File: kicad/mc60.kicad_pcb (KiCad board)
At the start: 2 copper layers, 60 x 70 mm, 108 parts, among them CN1 Conn_GPS, CN2 Conn_GNSS, CN3 SD_CARD, CN4 SIM_Card, CN5 Audio-Jack-4, CN6 5V_IN, J1 B_LS_N, J2 B_VRTC, J3 B_SPKP, J4 B_SPKN, J5 B_ADC, Q1 DTC114E, Q2 DTC114E, Q3 DTC114E, Q4 DTC143ZUA, U1 MC60_0, U2 TXB0108PWR, U3 MIC29302, U4 LP5907-3V3, U5 LP5907-2V8

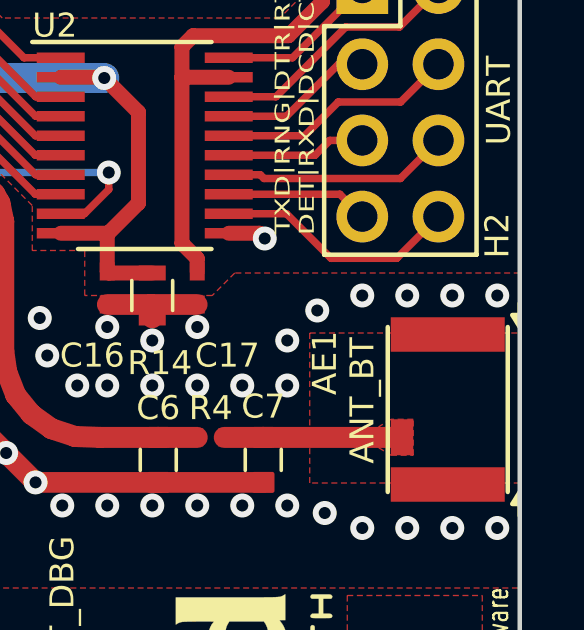
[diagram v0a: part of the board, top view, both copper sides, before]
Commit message: layout wip
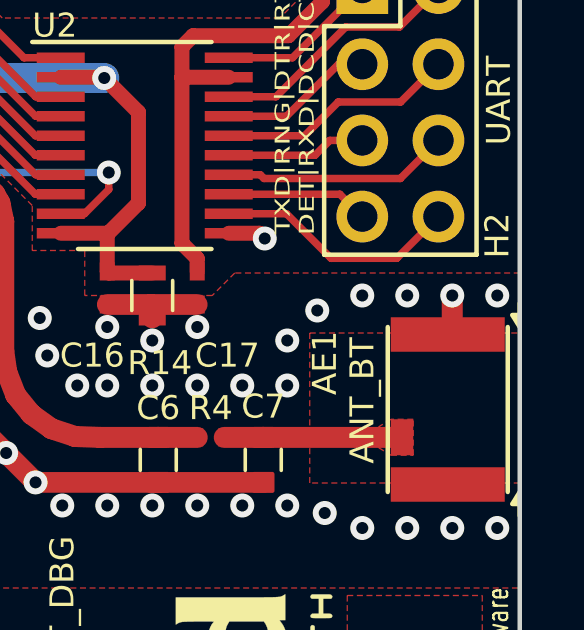
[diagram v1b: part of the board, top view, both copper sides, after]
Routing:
- net GND: track 272.8 -> 274.1 mm
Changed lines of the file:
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@@
-(kicad_pcb (version 20171130) (host pcbnew 5.0.0-rc2-dev-unknown-5d71153~64~ubuntu17.10.1)
+(kicad_pcb (version 20171130) (host pcbnew 5.0.0-rc2-dev-unknown-c8a7840~64~ubuntu16.04.1)
   (general
     (thickness 1.6)
     (drawings 25)
-    (tracks 1046)
+    (tracks 1048)
     (zones 0)
     (modules 108)
@@
     (0 F.Cu signal)
     (31 B.Cu signal)
-    (32 B.Adhes user hide)
-    (33 F.Adhes user hide)
+    (32 B.Adhes user)
+    (33 F.Adhes user)
     (34 B.Paste user hide)
     (35 F.Paste user hide)
     (36 B.SilkS user)
     (37 F.SilkS user)
-    (38 B.Mask user hide)
+    (38 B.Mask user)
     (39 F.Mask user)
     (40 Dwgs.User user)
@@
       (effects (font (size 0.8 0.8) (thickness 0.12)) (justify mirror))
     )
-    (fp_text value B_LS_N (at 0 -3.5 -90) (layer B.SilkS)
+    (fp_text value B_LS_N (at 0 -3.5 90) (layer B.SilkS)
       (effects (font (size 0.8 0.8) (thickness 0.12)) (justify mirror))
     )
@@
   (via (at 92.25 112.25) (size 0.7) (drill 0.4) (layers F.Cu B.Cu) (net 1))
   (segment (start 92.25 111.5) (end 92.25 112.25) (width 0.7) (layer F.Cu) (net 1))
+  (segment (start 126.75 108.15) (end 126.6 108.3) (width 0.7) (layer F.Cu) (net 1))
+  (segment (start 126.75 107) (end 126.75 108.15) (width 0.7) (layer F.Cu) (net 1))
   (segment (start 119.15 111.73) (end 120.45 111.73) (width 0.7) (layer F.Cu) (net 2) (status 30))
   (segment (start 125.07 111.73) (end 125.075 111.725) (width 0.7) (layer F.Cu) (net 2) (status 30))
